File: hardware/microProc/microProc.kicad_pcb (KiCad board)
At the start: 2 copper layers, 58 x 48.1 mm, 27 parts, among them J1 POWER, J2 INPUT, J3 OUTPUT, J4 Conn_02x07_Odd_Even, U1 STM32L021K4Tx, U2 BU33SD5WG-TR, U3 MCP4801

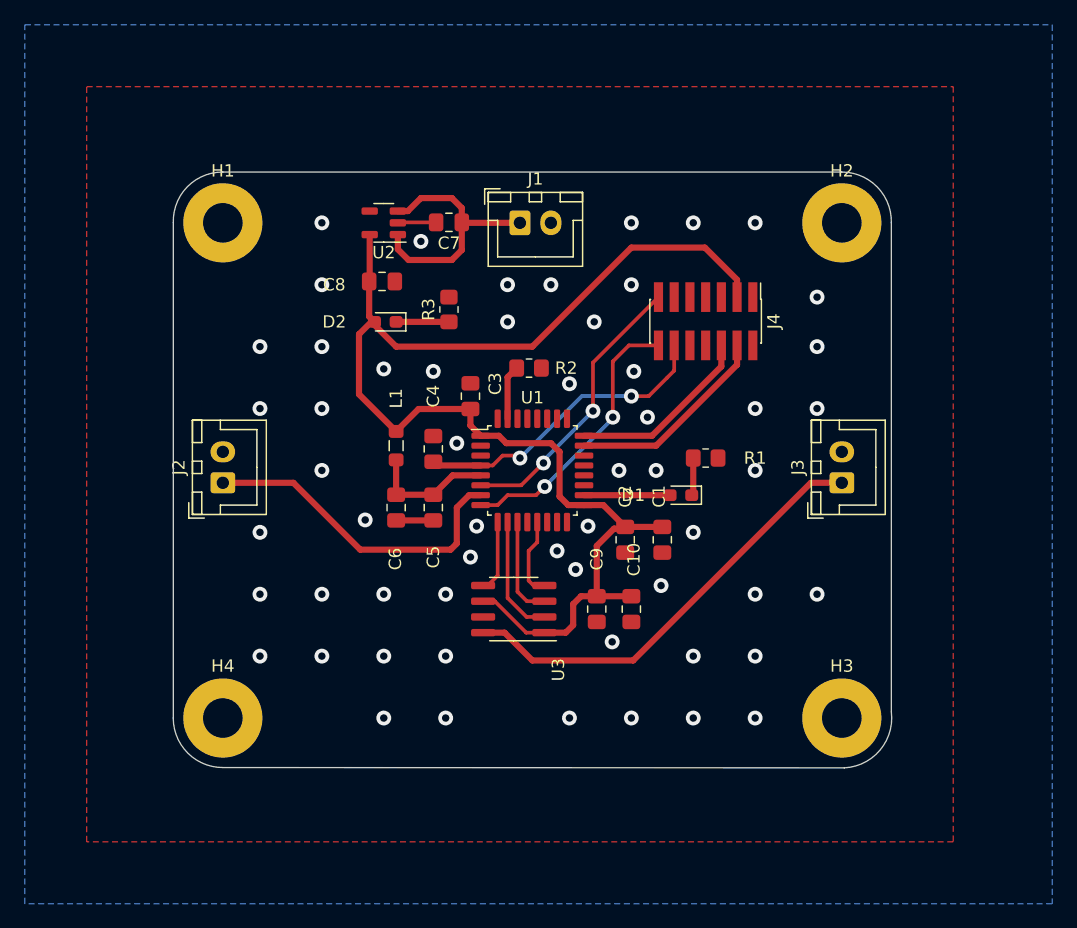
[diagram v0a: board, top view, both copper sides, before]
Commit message: Final Final PCB
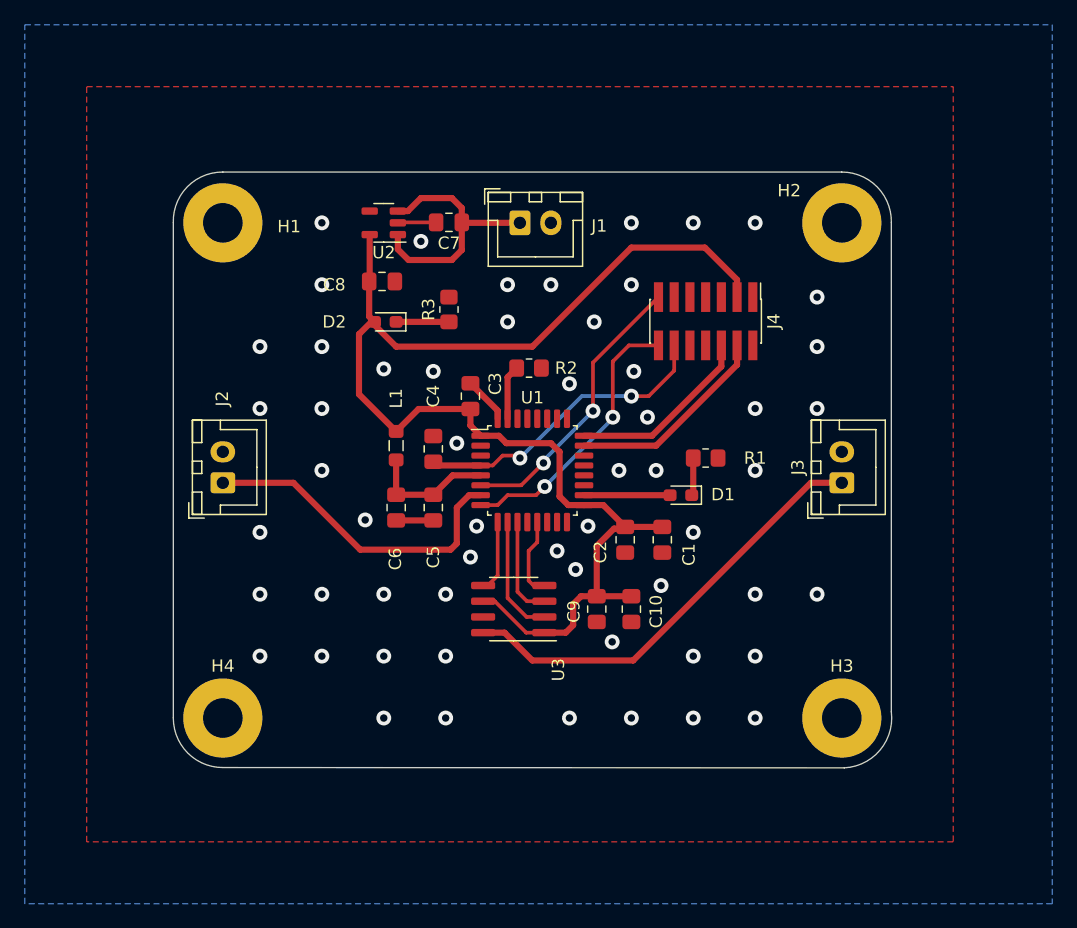
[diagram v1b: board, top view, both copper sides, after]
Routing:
- net GND: track 3.11 -> 6.88 mm
